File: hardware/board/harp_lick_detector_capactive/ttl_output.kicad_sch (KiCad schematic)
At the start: 8 parts

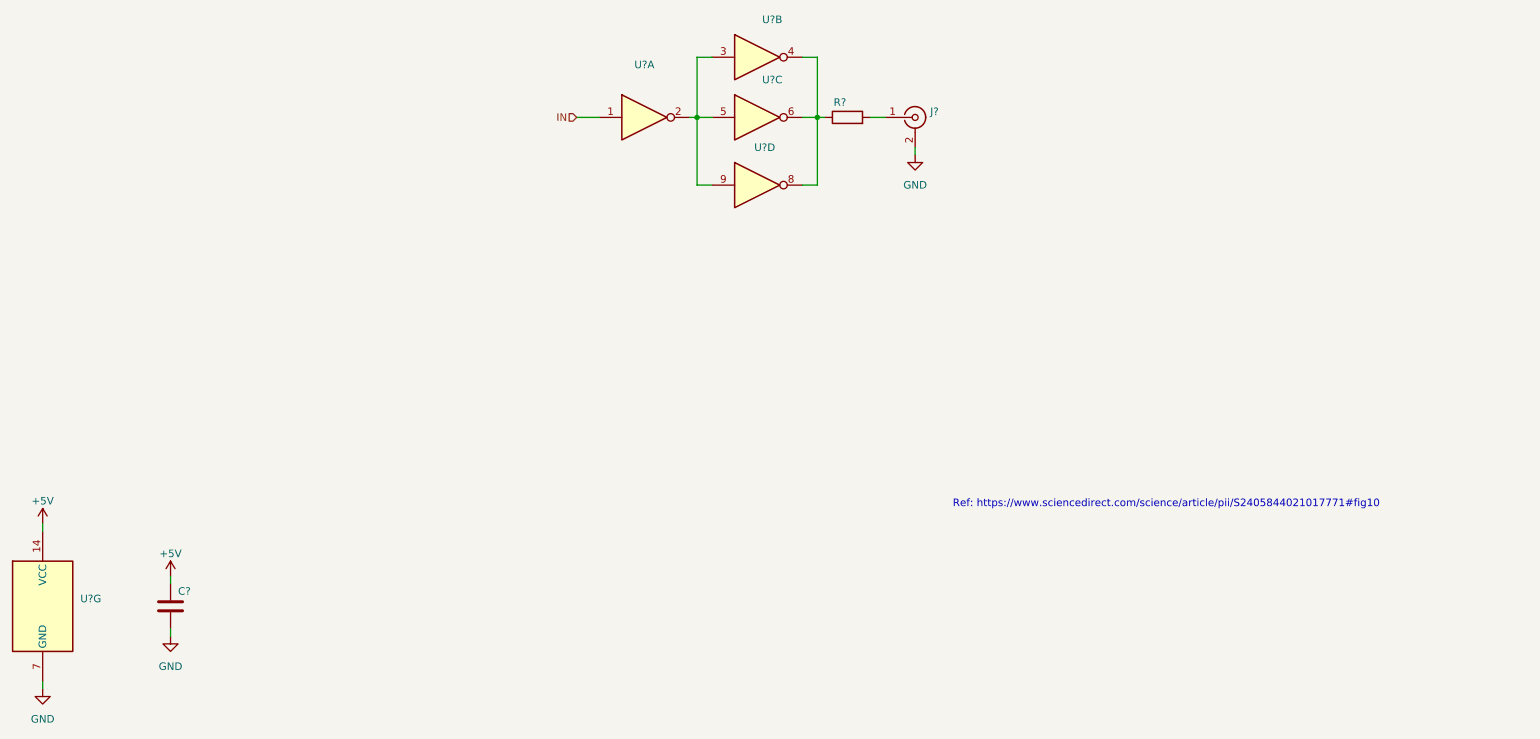
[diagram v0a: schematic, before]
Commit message: add driven shield
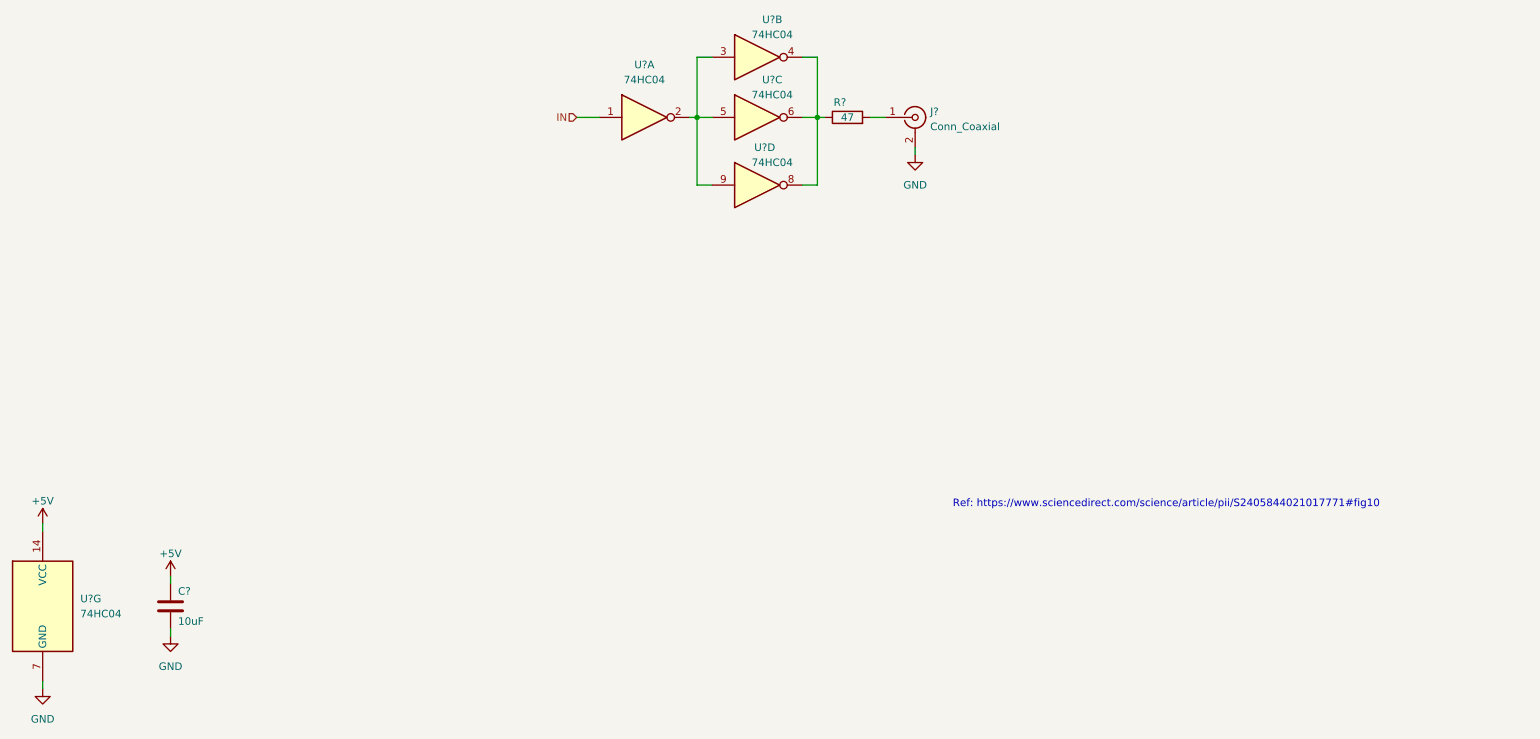
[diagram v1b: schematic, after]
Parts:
- C?: value (none) -> 10uF; footprint (none) -> Capacitor_SMD:C_0805_2012Metric
- J?: value (none) -> Conn_Coaxial
- R?: value (none) -> 47
- U? (x5): value (none) -> 74HC04
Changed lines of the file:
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@@
     (in_bom yes) (on_board yes)
     (property "Reference" "U?" (id 0) (at 147.32 85.09 0))
-    (property "Value" "" (id 1) (at 147.32 87.63 0))
+    (property "Value" "74HC04" (id 1) (at 147.32 87.63 0))
     (property "Footprint" "" (id 2) (at 144.78 91.44 0)
       (effects (font (size 1.27 1.27)) hide)
@@
       (effects (font (size 1.27 1.27)) (justify left))
     )
-    (property "Value" "" (id 1) (at 173.99 93.0031 0)
+    (property "Value" "Conn_Coaxial" (id 1) (at 173.99 93.0031 0)
       (effects (font (size 1.27 1.27)) (justify left))
     )
@@
     (in_bom yes) (on_board yes)
     (property "Reference" "U?" (id 0) (at 146.05 96.52 0))
-    (property "Value" "" (id 1) (at 147.32 99.06 0))
+    (property "Value" "74HC04" (id 1) (at 147.32 99.06 0))
     (property "Footprint" "" (id 2) (at 144.78 102.87 0)
       (effects (font (size 1.27 1.27)) hide)
@@
     (in_bom yes) (on_board yes)
     (property "Reference" "U?" (id 0) (at 147.32 74.93 0))
-    (property "Value" "" (id 1) (at 147.32 77.47 0))
+    (property "Value" "74HC04" (id 1) (at 147.32 77.47 0))
     (property "Footprint" "" (id 2) (at 144.78 81.28 0)
       (effects (font (size 1.27 1.27)) hide)
@@
       (effects (font (size 1.27 1.27)) (justify left))
     )
-    (property "Value" "" (id 1) (at 46.99 176.53 0)
-      (effects (font (size 1.27 1.27)) (justify left))
-    )
-    (property "Footprint" "" (id 2) (at 46.6852 177.8 0)
+    (property "Value" "10uF" (id 1) (at 46.99 176.53 0)
+      (effects (font (size 1.27 1.27)) (justify left))
+    )
+    (property "Footprint" "Capacitor_SMD:C_0805_2012Metric" (id 2) (at 46.6852 177.8 0)
       (effects (font (size 1.27 1.27)) hide)
     )
@@
       (effects (font (size 1.27 1.27)) (justify left))
     )
-    (property "Value" "" (id 1) (at 30.48 175.2599 0)
+    (property "Value" "74HC04" (id 1) (at 30.48 175.2599 0)
       (effects (font (size 1.27 1.27)) (justify left))
     )
@@
     (in_bom yes) (on_board yes)
     (property "Reference" "R?" (id 0) (at 158.75 88.9 90))
-    (property "Value" "" (id 1) (at 160.02 91.44 90))
+    (property "Value" "47" (id 1) (at 160.02 91.44 90))
     (property "Footprint" "" (id 2) (at 160.02 93.218 90)
       (effects (font (size 1.27 1.27)) hide)
@@
     (in_bom yes) (on_board yes) (fields_autoplaced)
     (property "Reference" "U?" (id 0) (at 125.73 82.55 0))
-    (property "Value" "" (id 1) (at 125.73 85.09 0))
+    (property "Value" "74HC04" (id 1) (at 125.73 85.09 0))
     (property "Footprint" "" (id 2) (at 125.73 91.44 0)
       (effects (font (size 1.27 1.27)) hide)
